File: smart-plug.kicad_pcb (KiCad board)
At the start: 2 copper layers, 58 x 53 mm, 31 parts, among them J1 Screw_Terminal_01x04, Q1 STGD5NB120SZ, Q2 BTA316B-600E, U1 THINGLER-ESP32-PICO, U2 SR086, U3 TPS560430X3F, U4 FODM3012, U5 LM4041, U6 ACS71240LLCBTR-030B3

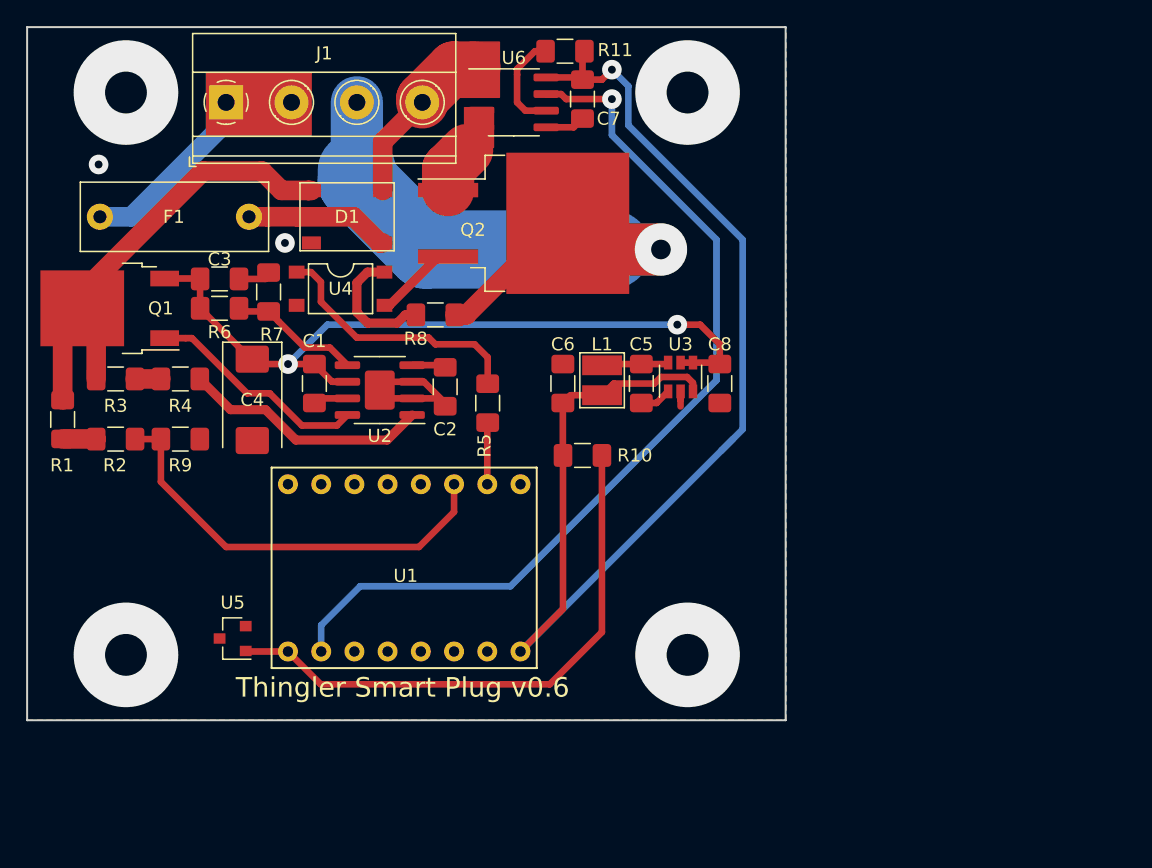
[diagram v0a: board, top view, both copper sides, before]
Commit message: Thingler 3D Smart Plug
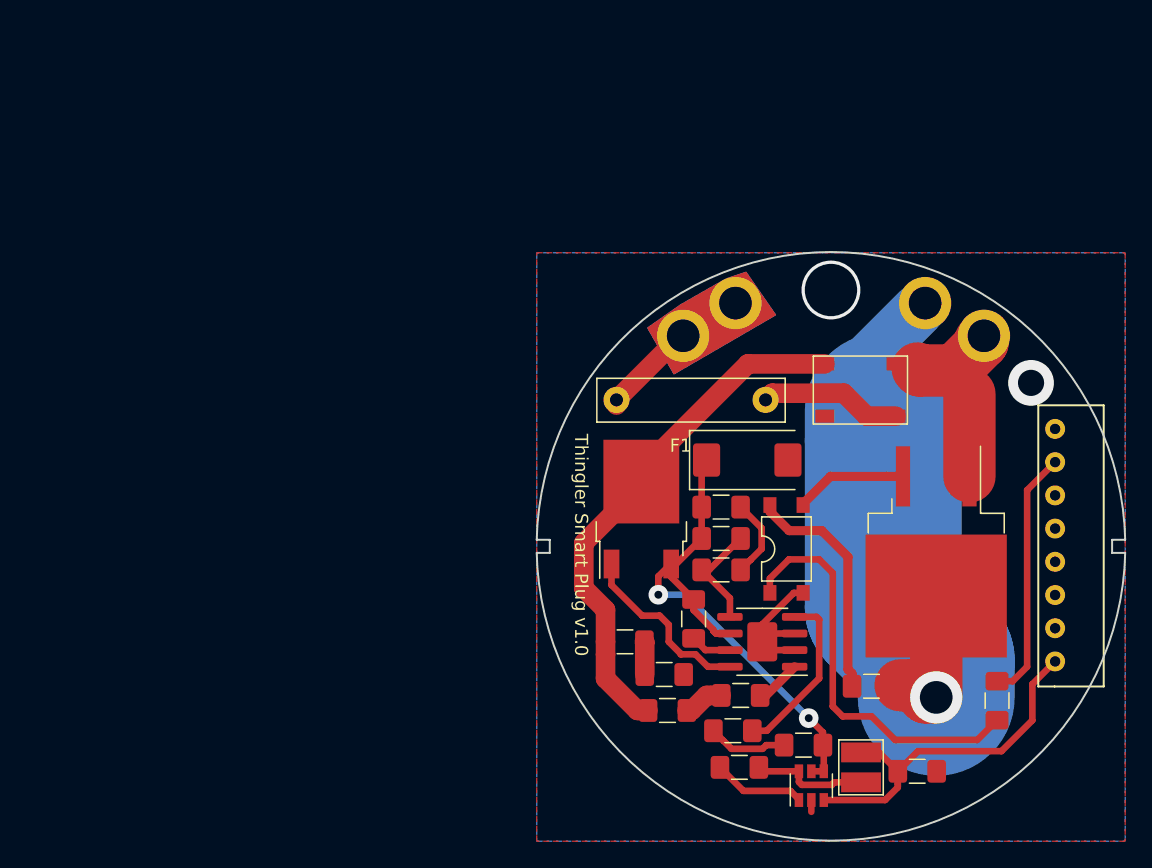
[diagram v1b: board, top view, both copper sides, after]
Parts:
- removed C8: 100n, Capacitor_SMD:C_1206_3216Metric_Pad1.42x1.75mm_HandSolder
- removed R10: 12.4k, Resistor_SMD:R_1206_3216Metric_Pad1.42x1.75mm_HandSolder
- removed R11: 113k, Resistor_SMD:R_1206_3216Metric_Pad1.42x1.75mm_HandSolder
- removed R9: 2.4k 0.1%, Resistor_SMD:R_1206_3216Metric_Pad1.42x1.75mm_HandSolder
- removed U5: LM4041, Package_TO_SOT_SMD:SOT-23
- removed U6: ACS71240LLCBTR-030B3, Package_SO:SOIC-8_3.9x4.9mm_P1.27mm
- C6: value 33u -> 100n
- C7: value 100n -> 33u
- J1: footprint TerminalBlock_Phoenix:TerminalBlock_Phoenix_MKDS-1,5-4_1x04_P5.00mm_Horizontal -> smart-plug:3d_power_connector
- R1, R2: value 200k 0.1% -> 200k
- U1: footprint smart-plug:THINGLER-ESP32-PICO -> smart-plug:Thingler-esp32-vertical
- U3: value TPS560430X3F -> FODM3012; footprint Package_TO_SOT_SMD:SOT-23-6 -> smart-plug:FODM3012
- U4: value FODM3012 -> TPS560430X3F; footprint smart-plug:FODM3012 -> Package_TO_SOT_SMD:SOT-23-6
- moved C7 57.4 mm to (184.1, 109.9), turned to 180 degrees
- moved U4 52.3 mm to (176.0, 111.0), turned to 90 degrees
- moved R3 49.2 mm to (165.0, 105.2)
- moved R4 49.2 mm to (170.6, 104.1)
- moved J1 48.9 mm to (177.7, 74.1)
- moved R1 46.2 mm to (161.8, 100.0), turned to 0 degrees
- moved R2 45.6 mm to (164.8, 102.5)
- moved R5 45.1 mm to (190.2, 104.5), turned to 90 degrees
- moved R8 43.8 mm to (180.6, 103.4)
- moved Q1 43.5 mm to (163.0, 89.8), turned to 90 degrees
- moved R6 42.2 mm to (169.1, 92.1)
- moved C3 42.1 mm to (169.1, 89.7)
- moved F1 41.9 mm to (172.5, 81.5)
- moved D1 41.4 mm to (179.8, 80.8)
- moved U1 40.9 mm to (194.6, 101.5), turned to 180 degrees
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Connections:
- C5 pad 1: Net-(C5-Pad1) -> /12VDC
- C5 pad 2: Net-(C5-Pad2) -> Earth
- C6 pad 1: Earth -> Net-(C6-Pad1)
- C6 pad 2: +3V3 -> Net-(C6-Pad2)
- C7 pad 1: +3V3 -> Earth
- C7 pad 2: Earth -> +3V3
- L1 pad 1: Net-(C5-Pad2) -> Net-(C6-Pad2)
- Q2 pad 1: Net-(Q2-Pad1) -> NEUT
- R2 pad 2: /I37 -> Earth
- U1 pad 7: /IO33 -> Net-(R5-Pad2)
- U1 pad 8: Net-(R10-Pad2) -> (no net)
- U3 pad 1: Net-(C5-Pad1) -> Net-(R5-Pad1)
- U3 pad 3: +3V3 -> Net-(Q2-Pad3)
- U3 pad 4: /12VDC -> Net-(R8-Pad2)
- U4 pad 1: Net-(R5-Pad1) -> Net-(C6-Pad1)
- U4 pad 3: Net-(Q2-Pad3) -> +3V3
- U4 pad 4: Net-(R8-Pad2) -> /12VDC
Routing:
- net /IO33: track 70.0 -> 0.00 mm, vias 1 -> 0
- net +3V3: track 97.4 -> 27.8 mm, vias 1 -> 0
- net Net-(R10-Pad2): track 43.5 -> 0.00 mm
- net /I37: track 33.0 -> 0.00 mm
- net /12VDC: track 58.0 -> 40.8 mm
- net Net-(R4-Pad2): track 19.0 -> 3.55 mm
- net Net-(R5-Pad2): track 4.72 -> 19.9 mm
- net Net-(C2-Pad1): track 2.59 -> 13.2 mm
- net Net-(R5-Pad1): track 20.8 -> 31.4 mm
- net Net-(J1-Pad3): track 50.2 -> 40.0 mm
- net Net-(C6-Pad2): track 0.00 -> 8.93 mm
- net Net-(R8-Pad2): track 9.82 -> 17.9 mm
- net Net-(R11-Pad1): track 7.77 -> 0.00 mm
- net Net-(C6-Pad1): track 0.00 -> 7.10 mm
- net AC: track 19.2 -> 12.4 mm
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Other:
- board size 58 x 53 mm -> 45 x 45 mm
- net class AC230V_HIGH_POWER: trace_width 4 -> 12
- board text added: "Thingler Smart Plug v1.0"
- board text removed: "Thingler Smart Plug v0.6"
